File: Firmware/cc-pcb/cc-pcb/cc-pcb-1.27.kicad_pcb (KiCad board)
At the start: 2 copper layers, 31.5 x 33.5 mm, 25 parts, among them CON1 BARREL_JACK, IC1 ATMEGA328P-A, P1 CONN_20, P10 SCK, P11 MISO, P2 CONN_2, P4 GND, P5 DTR, P6 TXD, P7 RXD, P8 RST, P9 MOSI, SW1 SRS

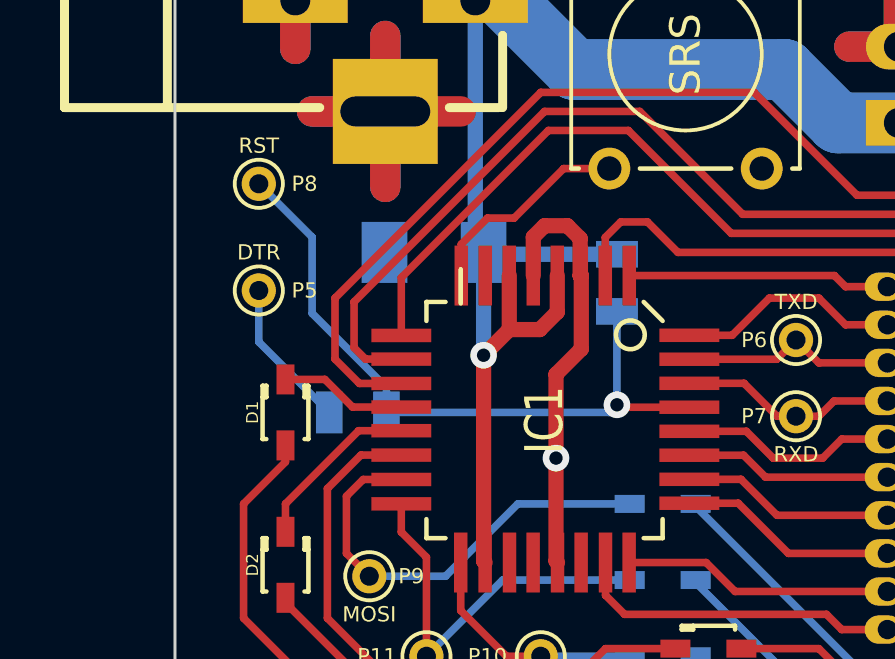
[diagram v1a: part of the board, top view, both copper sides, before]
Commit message: after dfm check
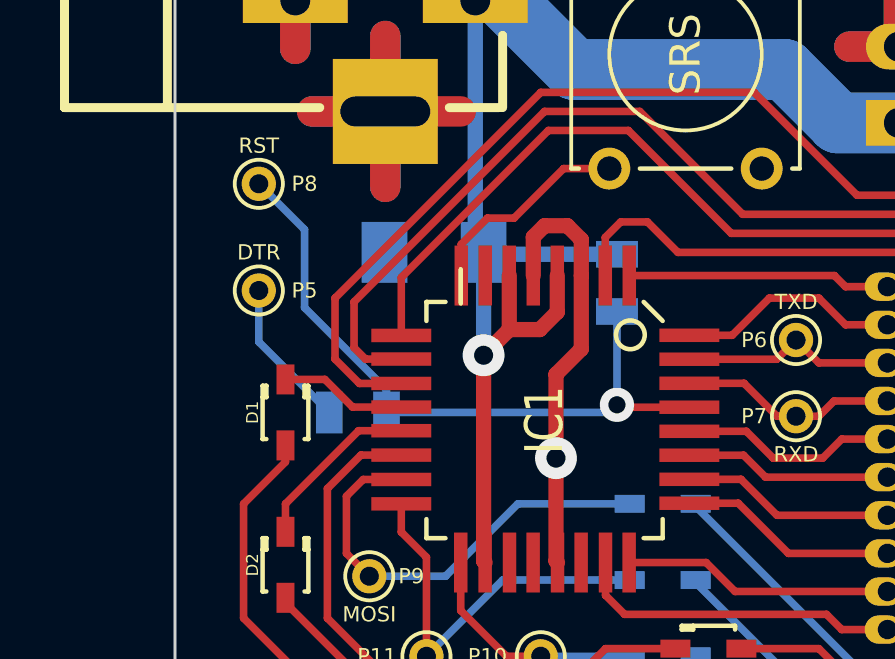
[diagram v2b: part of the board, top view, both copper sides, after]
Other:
- net class Default: via_dia 0.889 -> 1.143
- net class PWR: via_dia 0.889 -> 3.302; via_drill 0.635 -> 1.27
- net class PWRIC: via_dia 0.889 -> 1.397; via_drill 0.635 -> 0.889
- net class PWRTHR: via_dia 0.889 -> 2.032; via_drill 0.635 -> 1.016
